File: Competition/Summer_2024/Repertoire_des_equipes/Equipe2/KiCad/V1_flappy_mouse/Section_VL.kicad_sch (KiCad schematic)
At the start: 3 parts, among them J1 Conn_01x22_Pin, J2 Conn_01x22_Pin, J3 Conn_01x08_Pin

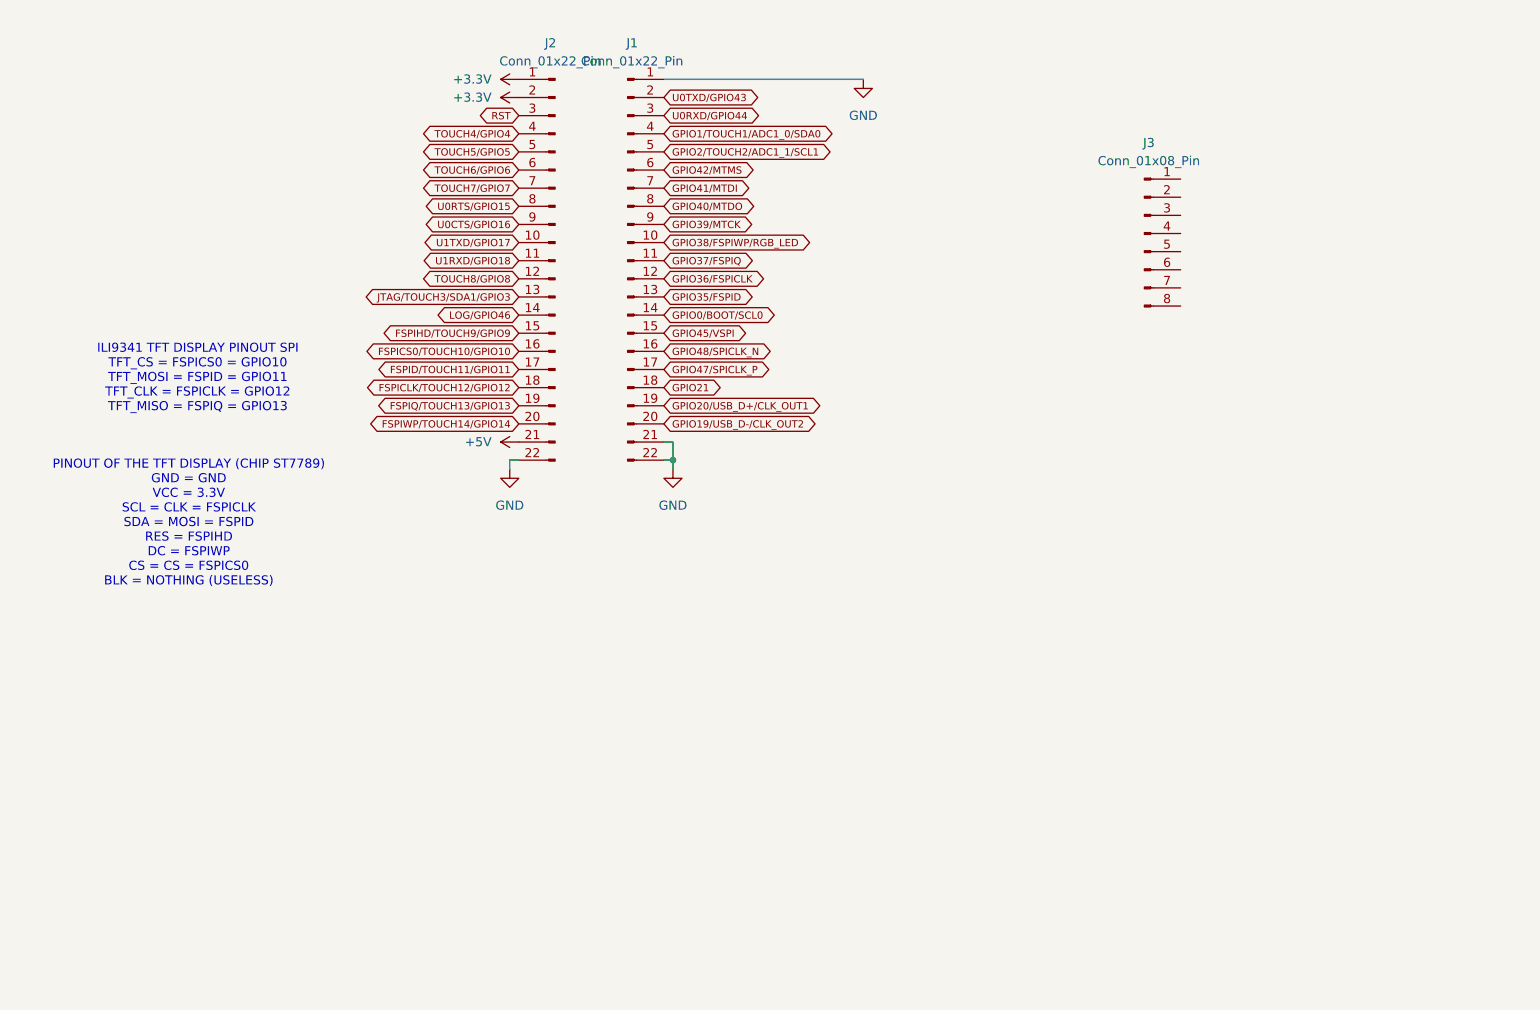
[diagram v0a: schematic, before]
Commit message: Revert "quick change"
This reverts commit a655ae3a92829bdf34a6315aef0ea8770937342e.
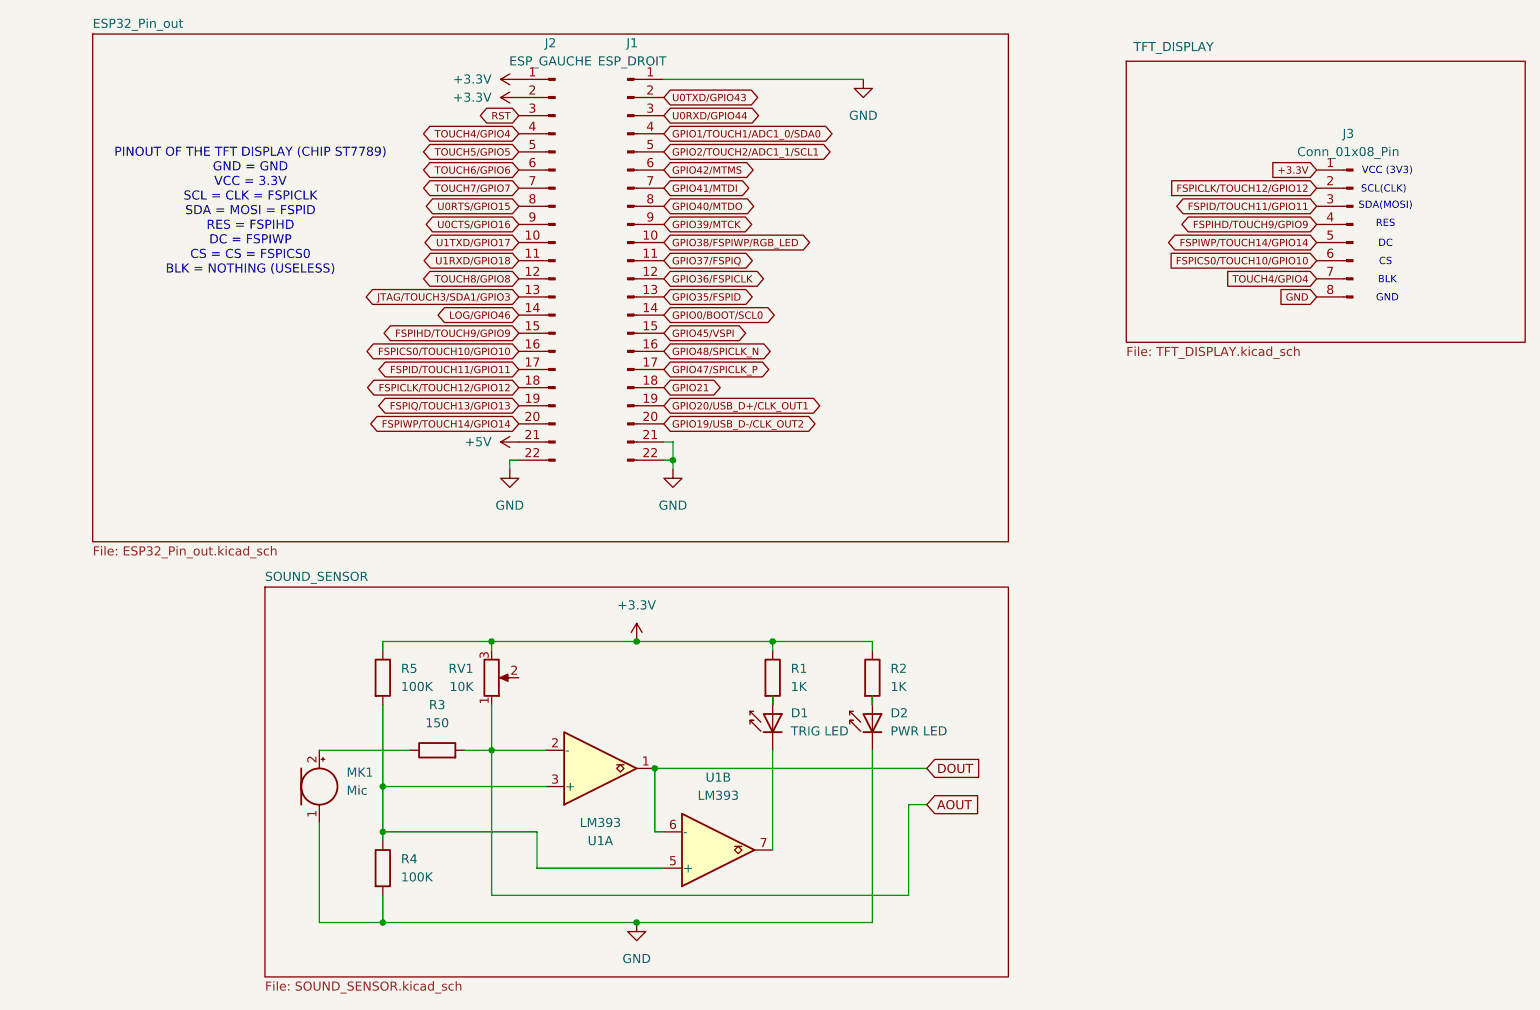
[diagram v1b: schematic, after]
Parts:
- added D1: TRIG LED, LED_THT:LED_D5.0mm_IRGrey, symbol LED:SFH4550
- added D2: PWR LED, LED_THT:LED_D5.0mm_IRGrey, symbol LED:SFH4550
- added MK1: Mic, symbol Device:Microphone
- added R1, R2: 1K, symbol Device:R
- added R3: 150, symbol Device:R
- added R4, R5: 100K, symbol Device:R
- added RV1: 10K, symbol Device:R_Potentiometer
- added U1: LM393, symbol Comparator:LM393
- J1: value Conn_01x22_Pin -> ESP_DROIT
- J2: value Conn_01x22_Pin -> ESP_GAUCHE
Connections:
- net +3.3V: now also J3.1 (Pin_1), R1.1, R2.1, R5.1, RV1.3
- net FSPICLK/TOUCH12/GPIO12: now also J3.2 (Pin_2)
- net FSPICS0/TOUCH10/GPIO10: now also J3.6 (Pin_6)
- net FSPID/TOUCH11/GPIO11: now also J3.3 (Pin_3)
- net FSPIHD/TOUCH9/GPIO9: now also J3.4 (Pin_4)
- net FSPIWP/TOUCH14/GPIO14: now also J3.5 (Pin_5)
- net GND: now also J3.8 (Pin_8), D2.1 (K), MK1.1 (-), R4.2
- net TOUCH4/GPIO4: now also J3.7 (Pin_7)
- new net: R4.1, R5.2, U1.3 (+), U1.5 (+)
- new net: MK1.2 (+), R3.1
- new net: D2.2 (A), R2.2
- new net: D1.2 (A), R1.2
- new net: D1.1 (K), U1.7
- new net AOUT: R3.2, RV1.1, U1.2 (-)
- new net DOUT: U1.1, U1.6 (-)
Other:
- added sheet ESP32_Pin_out (ESP32_Pin_out.kicad_sch)
- added sheet SOUND_SENSOR (SOUND_SENSOR.kicad_sch)
- added sheet TFT_DISPLAY (TFT_DISPLAY.kicad_sch)
- note added: "BLK"
- note added: "CS"
- note added: "DC"
- note added: "GND"
- note added: "RES"
- note added: "SCL(CLK)"
- note added: "SDA(MOSI)"
- note added: "VCC (3V3)"
- note removed: "ILI9341 TFT DISPLAY PINOUT SPI TFT_CS = FSPICS0 = GPIO10 TFT_MOSI = FSPID = GPIO11 TFT_CLK = FSPICLK = GPIO12 TFT_MISO = FSPIQ = GPIO13"

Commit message: quick change
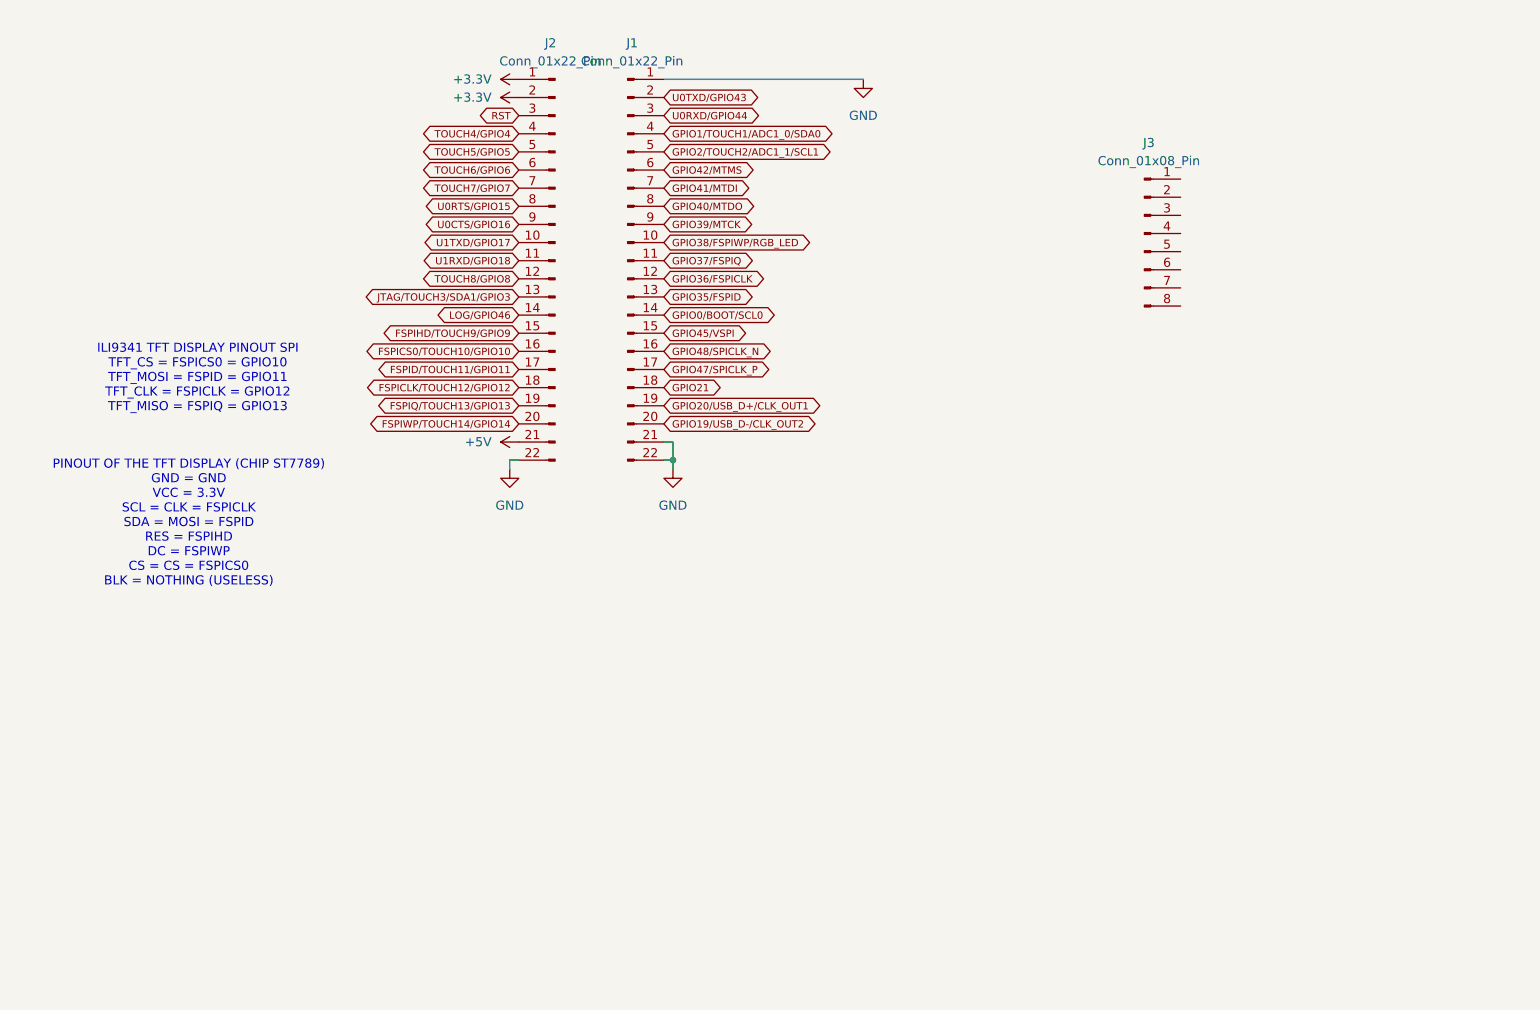
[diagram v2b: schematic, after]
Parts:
- removed D1: TRIG LED, LED_THT:LED_D5.0mm_IRGrey, symbol LED:SFH4550
- removed D2: PWR LED, LED_THT:LED_D5.0mm_IRGrey, symbol LED:SFH4550
- removed MK1: Mic, symbol Device:Microphone
- removed R1, R2: 1K, symbol Device:R
- removed R3: 150, symbol Device:R
- removed R4, R5: 100K, symbol Device:R
- removed RV1: 10K, symbol Device:R_Potentiometer
- removed U1: LM393, symbol Comparator:LM393
- J1: value ESP_DROIT -> Conn_01x22_Pin
- J2: value ESP_GAUCHE -> Conn_01x22_Pin
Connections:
- net +3.3V: no longer J3.1 (Pin_1)
- net FSPICLK/TOUCH12/GPIO12: no longer J3.2 (Pin_2)
- net FSPICS0/TOUCH10/GPIO10: no longer J3.6 (Pin_6)
- net FSPID/TOUCH11/GPIO11: no longer J3.3 (Pin_3)
- net FSPIHD/TOUCH9/GPIO9: no longer J3.4 (Pin_4)
- net FSPIWP/TOUCH14/GPIO14: no longer J3.5 (Pin_5)
- net GND: no longer J3.8 (Pin_8)
- net TOUCH4/GPIO4: no longer J3.7 (Pin_7)
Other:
- removed sheet ESP32_Pin_out
- removed sheet SOUND_SENSOR
- removed sheet TFT_DISPLAY
- note added: "ILI9341 TFT DISPLAY PINOUT SPI TFT_CS = FSPICS0 = GPIO10 TFT_MOSI = FSPID = GPIO11 TFT_CLK = FSPICLK = GPIO12 TFT_MISO = FSPIQ = GPIO13"
- note removed: "BLK"
- note removed: "CS"
- note removed: "DC"
- note removed: "GND"
- note removed: "RES"
- note removed: "SCL(CLK)"
- note removed: "SDA(MOSI)"
- note removed: "VCC (3V3)"
